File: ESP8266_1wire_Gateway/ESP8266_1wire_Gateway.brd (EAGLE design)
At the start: 44 x 44 mm, 72 parts, among them IC1 5V, IC2 3.3V, IC3 DS2482-100S, IC4 DS18B20, Q1 BSS84, Q2 BSS138, Q3 BSS138

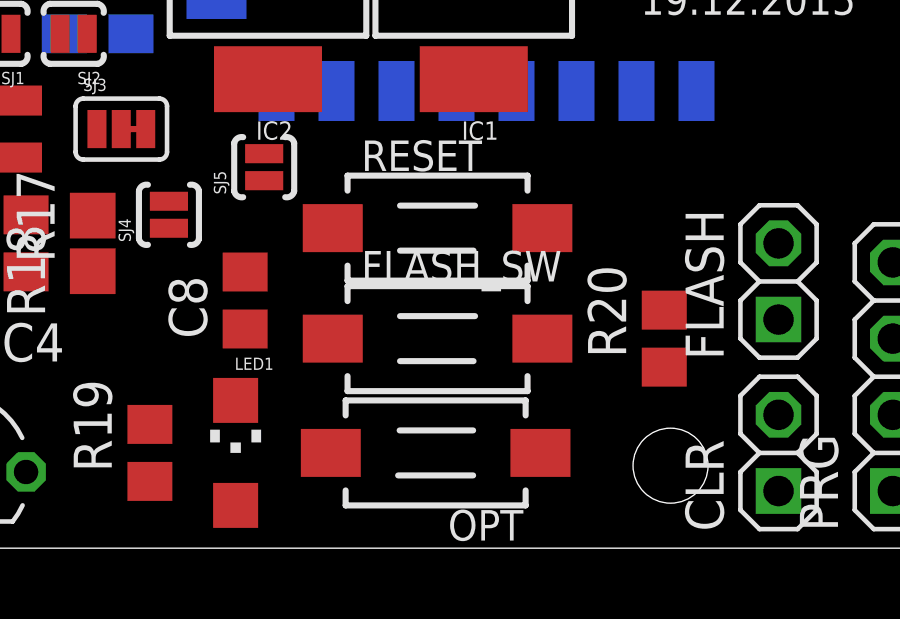
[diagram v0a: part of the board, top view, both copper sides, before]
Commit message: .
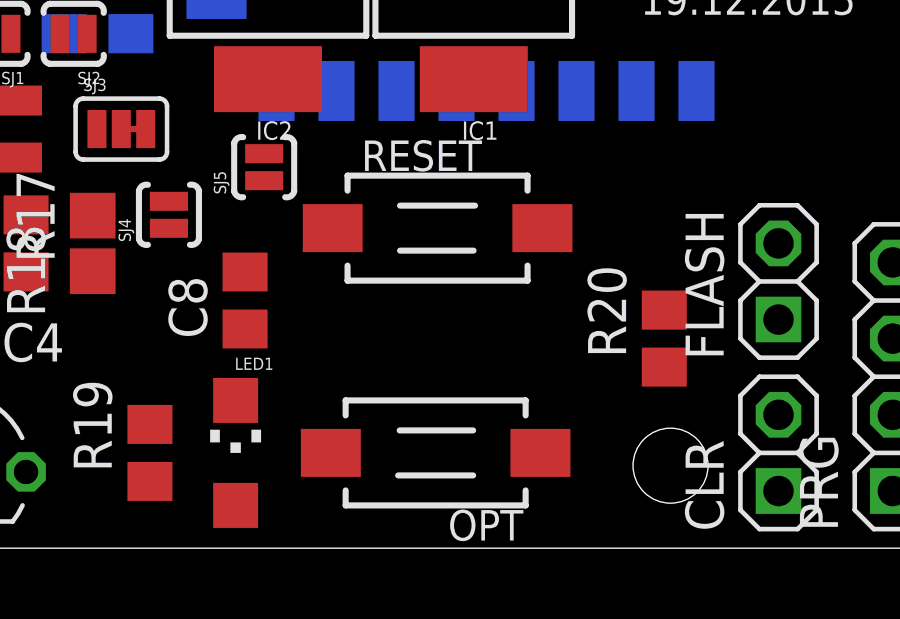
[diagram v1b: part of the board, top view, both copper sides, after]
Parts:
- removed FLASH_SW: DTSM-3, mechanics:DTSM-3
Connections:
- net GND: no longer FLASH_SW.2
- net N$10: no longer FLASH_SW.1
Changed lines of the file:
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@@
 <element name="R14" library="resistor" package="R0805" value="4k7" x="11.1125" y="31.4325" rot="MR90"/>
 <element name="R13" library="resistor" package="R0805" value="4k7" x="14.2875" y="18.0975" rot="MR90"/>
-<element name="FLASH_SW" library="mechanics" package="DTSM-3" value="DTSM-3" x="26.7335" y="6.985" smashed="yes">
-<attribute name="NAME" x="24.1935" y="8.89" size="1.016" layer="25" ratio="14"/>
-</element>
 <element name="U$1" library="ohw-logo" package="OSHW_FILLX100_NOTEXT" value="" x="43.4275" y="34.5375" rot="MR0"/>
 <element name="IC2" library="SparkFun-PowerIC" package="SOT223" value="3.3V" x="21.082" y="18.7325" smashed="yes" rot="R180">
@@
 <contactref element="RESET" pad="1"/>
 <contactref element="C3" pad="2"/>
-<contactref element="FLASH_SW" pad="2"/>
 <contactref element="C6" pad="2"/>
 <contactref element="IC2" pad="1"/>
@@
 <wire x1="23.1762" y1="3.175" x2="20.32" y2="9.205" width="0" layer="19" extent="1-1"/>
 <wire x1="20.0025" y1="1.425" x2="23.1762" y2="3.175" width="0" layer="19" extent="1-1"/>
-<wire x1="30.2273" y1="6.985" x2="23.2397" y2="10.668" width="0" layer="19" extent="1-1"/>
-<wire x1="41.91" y1="9.525" x2="30.2273" y2="6.985" width="0" layer="19" extent="1-1"/>
-<wire x1="38.1" y1="7.62" x2="20.0025" y2="1.425" width="0" layer="19" extent="1-1"/>
+<wire x1="38.1" y1="7.62" x2="23.2397" y2="10.668" width="0" layer="19" extent="1-1"/>
+<wire x1="41.91" y1="9.525" x2="38.1" y2="7.62" width="0" layer="19" extent="1-1"/>
 </signal>
 <signal name="N$1">
@@
 <signal name="N$10">
 <contactref element="FLASH" pad="2"/>
-<contactref element="FLASH_SW" pad="1"/>
 <contactref element="R12" pad="1"/>
-<wire x1="13.0175" y1="9.21" x2="23.2397" y2="6.985" width="0" layer="19" extent="1-1"/>
-<wire x1="38.1" y1="10.16" x2="13.0175" y2="9.21" width="0" layer="19" extent="1-1"/>
+<wire x1="13.0175" y1="9.21" x2="38.1" y2="10.16" width="0" layer="19" extent="1-1"/>
 </signal>
 </signals>

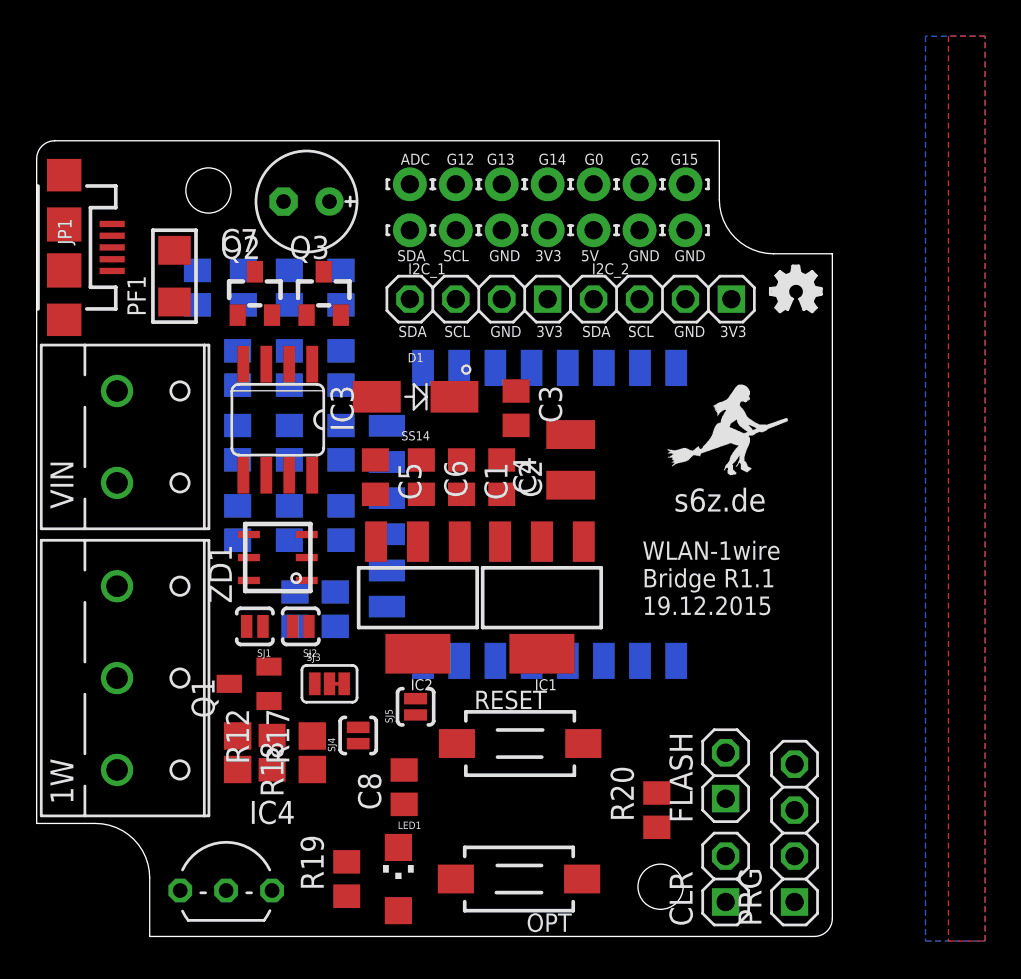
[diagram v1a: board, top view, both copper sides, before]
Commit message: v0.9
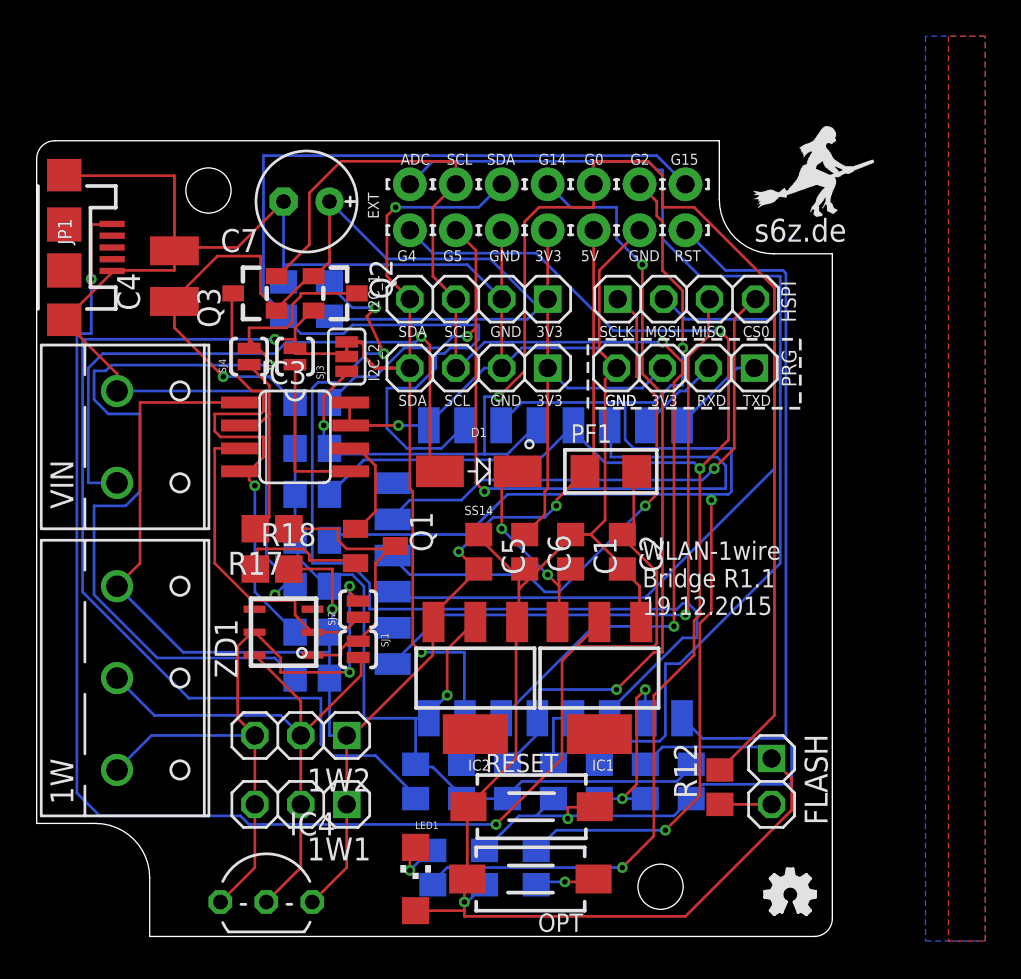
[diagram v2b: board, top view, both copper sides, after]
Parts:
- removed CLR: (no value), my:1X02
- removed G12, G13: LSP10, my:LSP10
- added 1W1, 1W2: (no value), my:1X03
- added G4, G5: LSP10, my:LSP10
- added HSPI: (no value), my:1X04
- RST: value GND -> RST
- moved R1 33.5 mm to (36.2, 8.57)
- moved U$1 33.3 mm to (43.1, 1.20)
- moved U$2 33.3 mm to (40.3, 1.20)
- moved R3 32.2 mm to (28.6, 8.57)
- moved PF1 26.4 mm to (31.8, 25.7), turned to 0 degrees
- moved PRG 26.4 mm to (35.9, 31.4), turned to 180 degrees
- moved R14 26.0 mm to (23.5, 8.57), turned to 270 degrees
- moved R12 24.8 mm to (37.8, 8.26)
- moved R10 24.6 mm to (31.1, 8.57)
- moved C4 24.1 mm to (7.62, 36.5)
- moved SJ4 21.8 mm to (11.7, 32.1)
- moved SJ5 20.5 mm to (14.3, 32.1)
- moved R11 19.6 mm to (33.7, 8.57)
- moved R7 18.7 mm to (26.0, 8.57)
- moved SJ3 18.1 mm to (17.1, 32.1), turned to 90 degrees
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- renumbered GND8 to RST
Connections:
- net CSN renamed GPIO15
- removed net GPIO0: G0.1, MDL1.12, R12.2, R5.1
- removed net GPIO2: G2.1, MDL1.11, R4.1, SJ3.1
- new net 1WDIR: G0.1, MDL1.12, R12.2, R5.1, SJ3.1
- new net GPIO5: G5.1, MDL1.14, R8.1
- new net HCS0: HSPI.4, MDL1.17
- new net HMISO: HSPI.3, MDL1.18
- new net HMOSI: HSPI.2, MDL1.21
- new net HSCLK: HSPI.1, MDL1.22
- net 1W_ESD: now also 1W1.2, 1W2.2
- net GND: no longer RST.1
- net GND_ESD: now also 1W1.3, 1W2.3
- net LED_OPT: now also G4.1, MDL1.13, R9.1; no longer G12.1, MDL1.6, R8.1
- net RST: now also RST.1
- net RXD: no longer CLR.2
- net SCL1: now also MDL1.6; no longer MDL1.14
- net SDA1: now also MDL1.7; no longer MDL1.13
- net SW_OPT: now also G2.1, MDL1.11, R4.1; no longer G13.1, MDL1.7, R9.1
- net TXD: no longer CLR.1
- net VCC_5V: now also 1W1.1, 1W2.1
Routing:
- net GND: track 0.00 -> 204.1 mm, vias 0 -> 3
- net VCC: track 0.00 -> 128.6 mm, vias 0 -> 2
- net VCC_5V: track 0.00 -> 89.1 mm, vias 0 -> 3
- net 5V_IN: track 0.00 -> 86.9 mm, vias 0 -> 2
- net LED_OPT: track 0.00 -> 86.1 mm, vias 0 -> 3
- net SW_OPT: track 0.00 -> 84.2 mm, vias 0 -> 3
- net 1WDIR: track 0.00 -> 80.2 mm, vias 0 -> 2
- net SCL1: track 0.00 -> 70.3 mm, vias 0 -> 2
- net RST: track 0.00 -> 63.4 mm, vias 0 -> 1
- net SDA2: track 0.00 -> 60.4 mm, vias 0 -> 1
- net GPIO15: track 0.00 -> 59.7 mm
- net N$5: track 0.00 -> 58.7 mm
- net SDA1X: track 0.00 -> 56.3 mm, vias 0 -> 1
- net CH_PD: track 0.00 -> 52.5 mm, vias 0 -> 2
- net GPIO5: track 0.00 -> 47.9 mm, vias 0 -> 2
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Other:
- board text added: "CS0"
- board text added: "EXT"
- board text added: "MISO"
- board text added: "MOSI"
- board text added: "RST"
- board text added: "RXD"
- board text added: "SCLK"
- board text added: "TXD"
